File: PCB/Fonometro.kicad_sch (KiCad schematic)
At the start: 58 parts, among them J1 Conn_01x15_Male, J2 Conn_01x15_Male, J3 Power, U1 LM324, U2 LM358, U3 ESP32-DEVKIT-V1

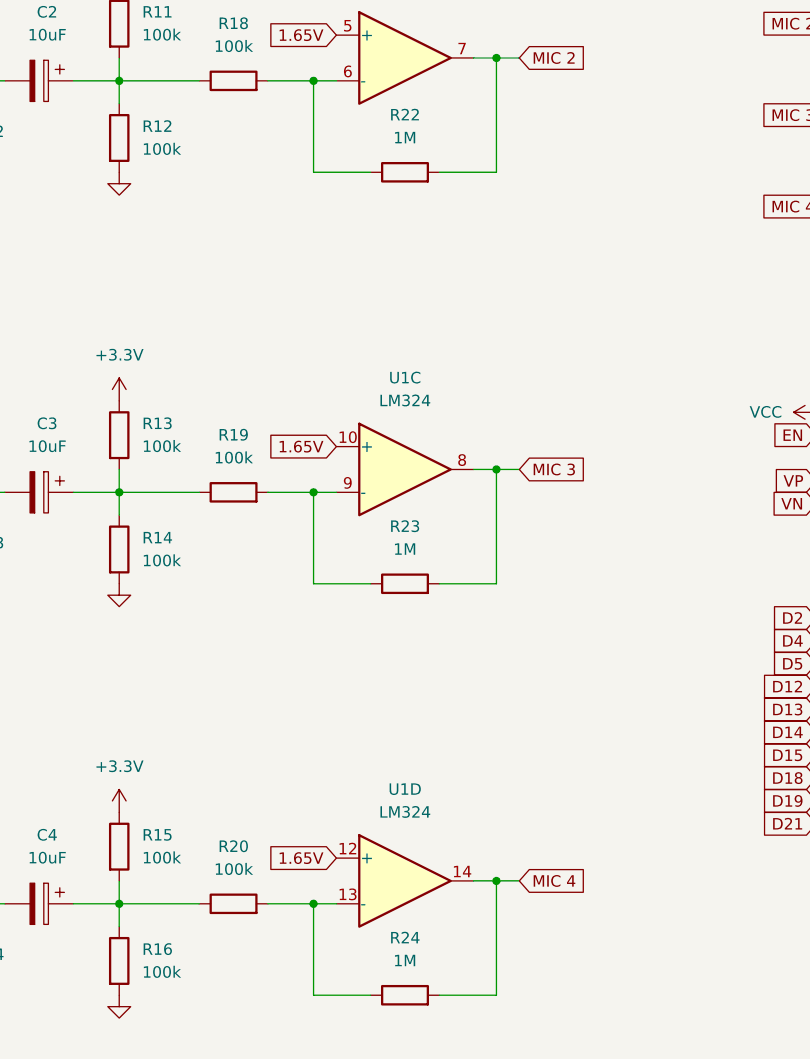
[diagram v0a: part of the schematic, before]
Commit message: feat: improved PCB layout.
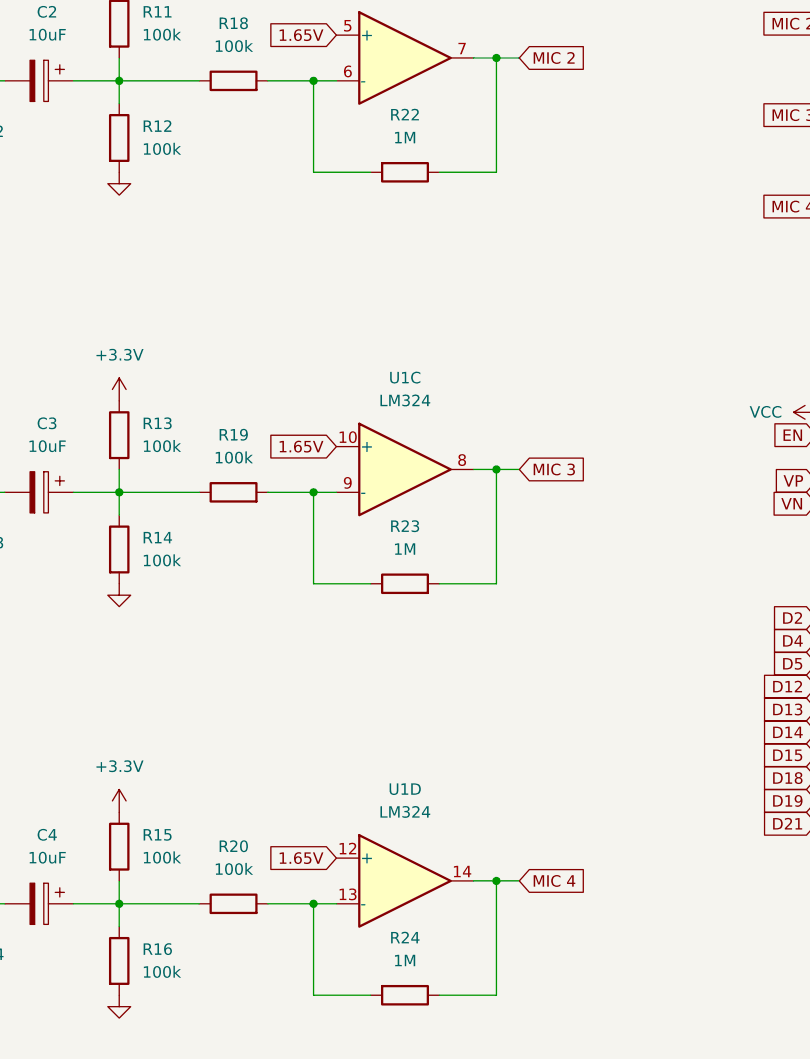
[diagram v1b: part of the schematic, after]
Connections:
- net MIC 2: now also R22.1; no longer R22.2
- net MIC 4: now also R24.1; no longer R24.2
- net at R20.2, U1.13 (-): now also R24.2; no longer R24.1
- net at R18.2, U1.6 (-): now also R22.2; no longer R22.1
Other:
- moved on the sheet: R22, R24
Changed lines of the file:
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@@
     (pin "1")
   )
-  (symbol (lib_id "Device:R") (at 73.66 96.52 90) (unit 1)
+  (symbol (lib_id "Device:R") (at 73.66 96.52 270) (unit 1)
     (in_bom yes) (on_board yes) (fields_autoplaced)
     (property "Reference" "R22" (id 0) (at 73.66 90.17 90))
     (property "Value" "1M" (id 1) (at 73.66 92.71 90))
-    (property "Footprint" "Resistor_THT:R_Axial_DIN0207_L6.3mm_D2.5mm_P7.62mm_Horizontal" (id 2) (at 73.66 98.298 90)
+    (property "Footprint" "Resistor_THT:R_Axial_DIN0207_L6.3mm_D2.5mm_P7.62mm_Horizontal" (id 2) (at 73.66 94.742 90)
       (effects (font (size 1.27 1.27)) hide)
     )
@@
     (pin "2")
   )
-  (symbol (lib_id "Device:R") (at 73.66 187.96 90) (unit 1)
+  (symbol (lib_id "Device:R") (at 73.66 187.96 270) (unit 1)
     (in_bom yes) (on_board yes) (fields_autoplaced)
     (property "Reference" "R24" (id 0) (at 73.66 181.61 90))
     (property "Value" "1M" (id 1) (at 73.66 184.15 90))
-    (property "Footprint" "Resistor_THT:R_Axial_DIN0207_L6.3mm_D2.5mm_P7.62mm_Horizontal" (id 2) (at 73.66 189.738 90)
+    (property "Footprint" "Resistor_THT:R_Axial_DIN0207_L6.3mm_D2.5mm_P7.62mm_Horizontal" (id 2) (at 73.66 186.182 90)
       (effects (font (size 1.27 1.27)) hide)
     )
